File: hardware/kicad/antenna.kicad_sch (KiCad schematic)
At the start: 44 parts, among them J5 BWIPX-1-001E, J7 BWIPX-1-001E, U14 SKY13414-485LF, U16 SKY13414-485LF

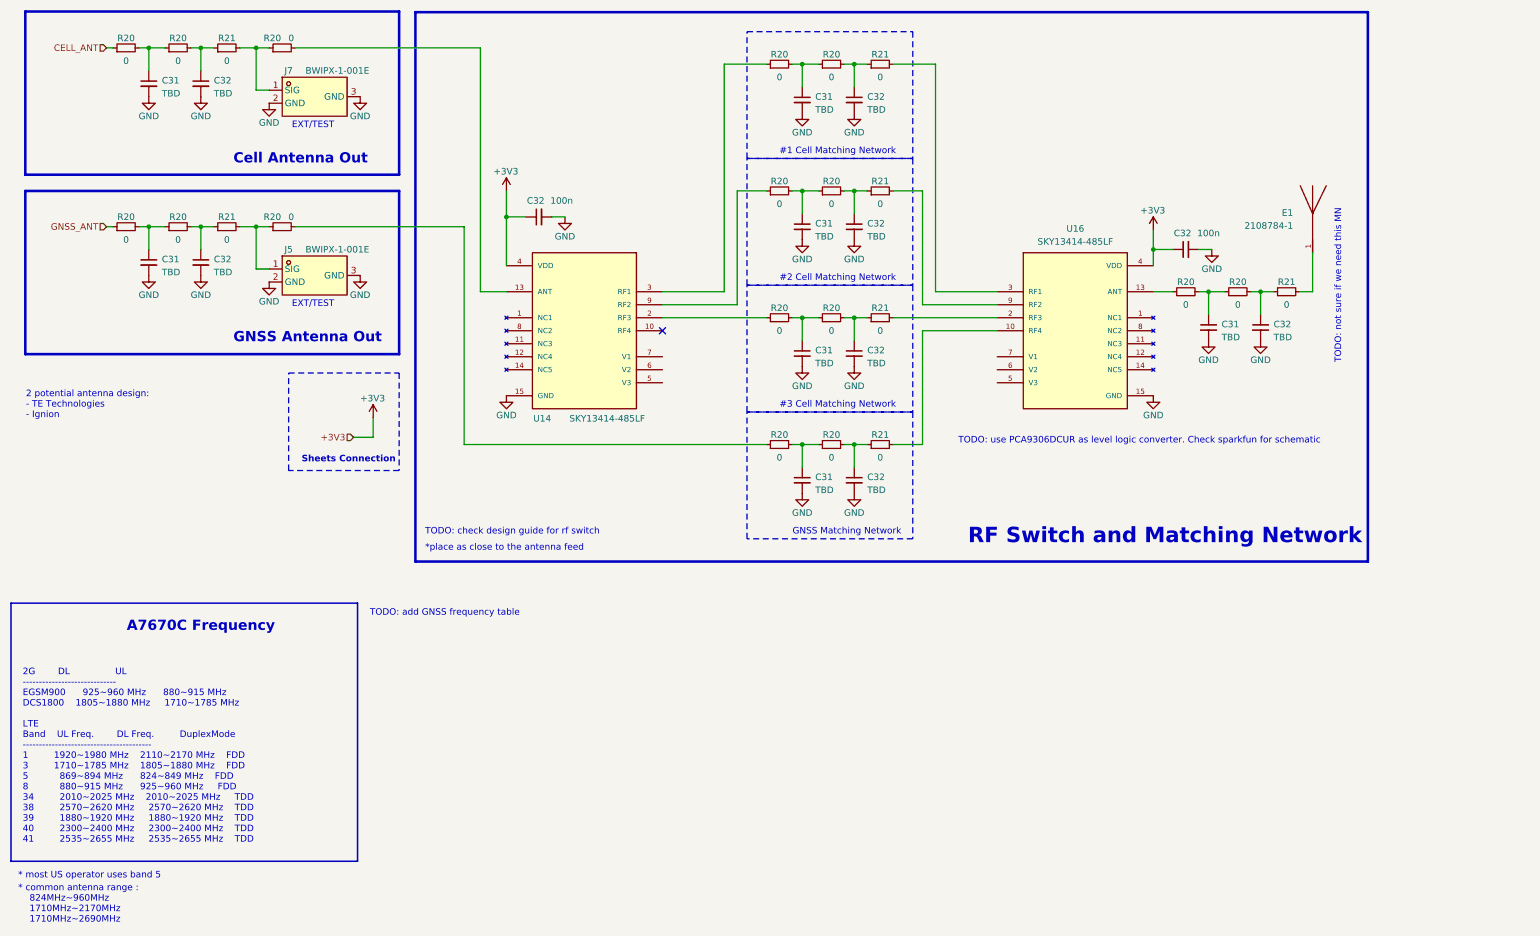
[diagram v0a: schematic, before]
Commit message: ignion antenna design
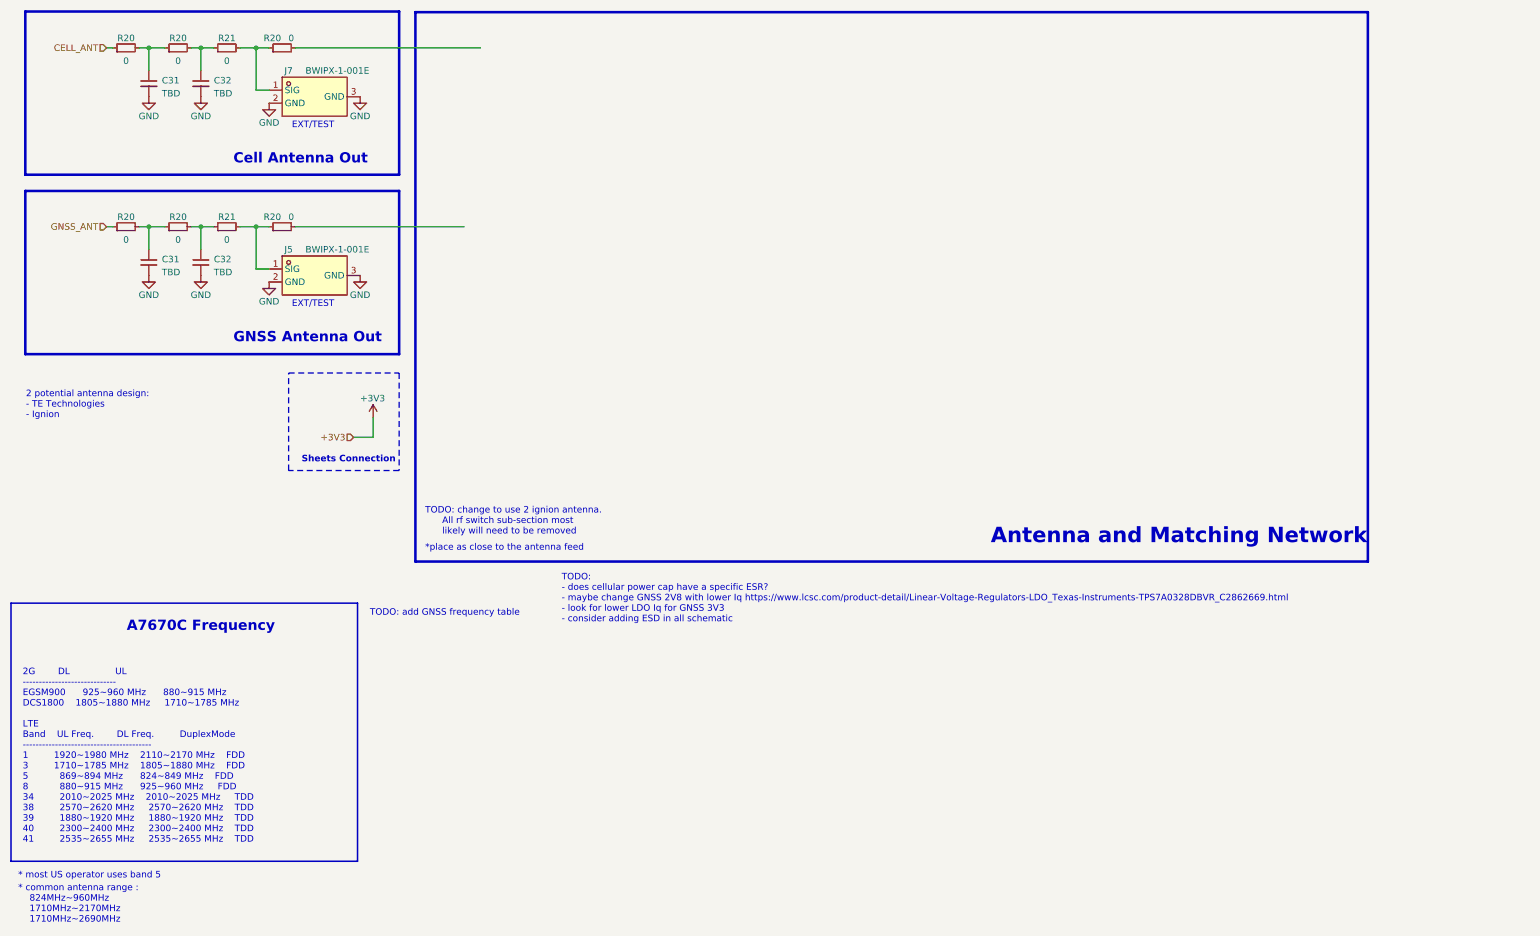
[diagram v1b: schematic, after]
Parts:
- removed C31 (x5), C32 (x5): TBD, Capacitor_SMD:C_0402_1005Metric, symbol Device:C_Small
- removed C32 (x2): 100n, Capacitor_SMD:C_0402_1005Metric, symbol Device:C_Small
- removed E1: 2108784-1, bwlc1a:2108784-1, symbol bwlc1a:2108784-1
- removed R20 (x10), R21 (x5): 0, Resistor_SMD:R_0402_1005Metric, symbol Device:R_Small
- removed U14, U16: SKY13414-485LF, symbol bwlc1a:SKY13414-485LF
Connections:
- no-connect marks 1 -> 0
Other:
- note added: "Antenna and Matching Network"
- note added: "TODO: - does cellular power cap have a specific ESR? - maybe change GNSS 2V8 with lower Iq https://www.lcsc.com/product-detail/Linear-Voltage-Regulators-LDO_Texas-Instruments-TPS7A0328DBVR_C2862669.html - look for lower LDO Iq for GNSS 3V3 - consider adding ESD in all schematic"
- note added: "TODO: change to use 2 ignion antenna. All rf switch sub-section most likely will need to be removed"
- note removed: "#1 Cell Matching Network"
- note removed: "#2 Cell Matching Network"
- note removed: "#3 Cell Matching Network"
- note removed: "GNSS Matching Network"
- note removed: "RF Switch and Matching Network"
- note removed: "TODO: check design guide for rf switch"
- note removed: "TODO: not sure if we need this MN"
- note removed: "TODO: use PCA9306DCUR as level logic converter. Check sparkfun for schematic"
